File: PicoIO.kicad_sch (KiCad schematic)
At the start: 14 parts

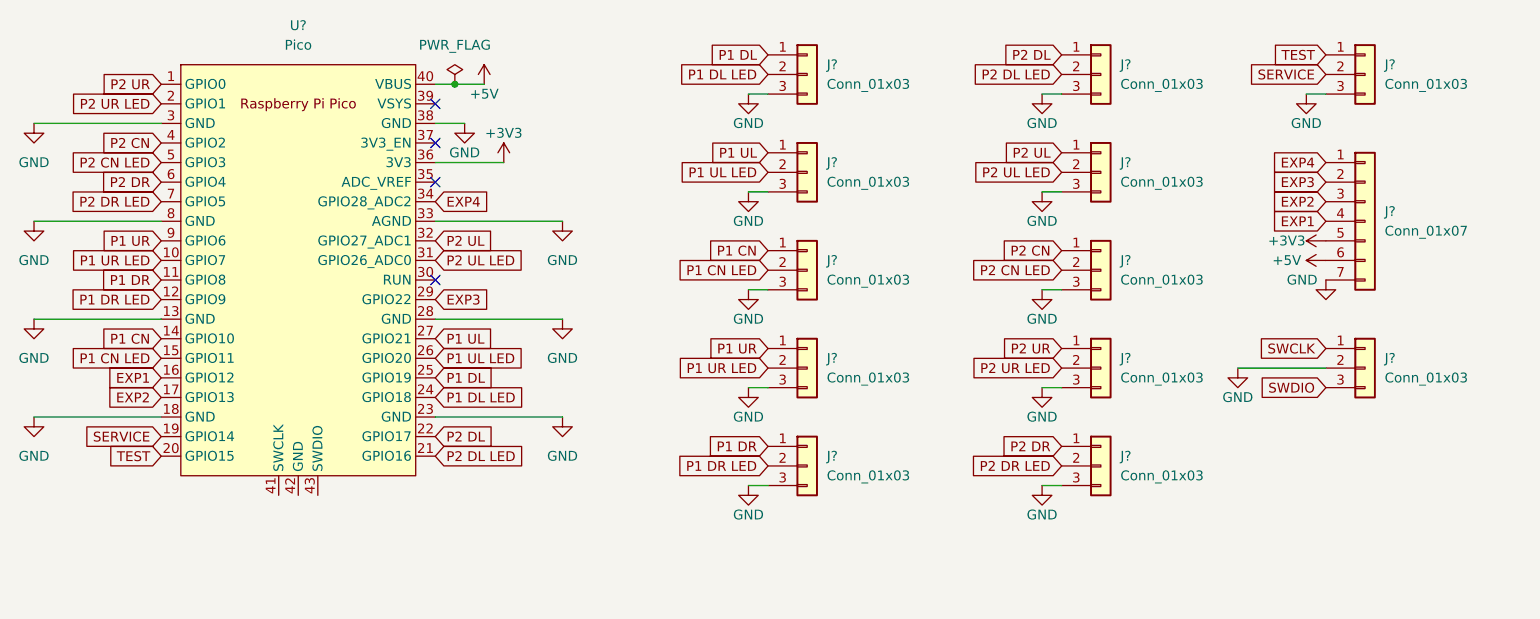
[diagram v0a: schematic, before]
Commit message: PCB revision 1 (NOT READY FOR USE)
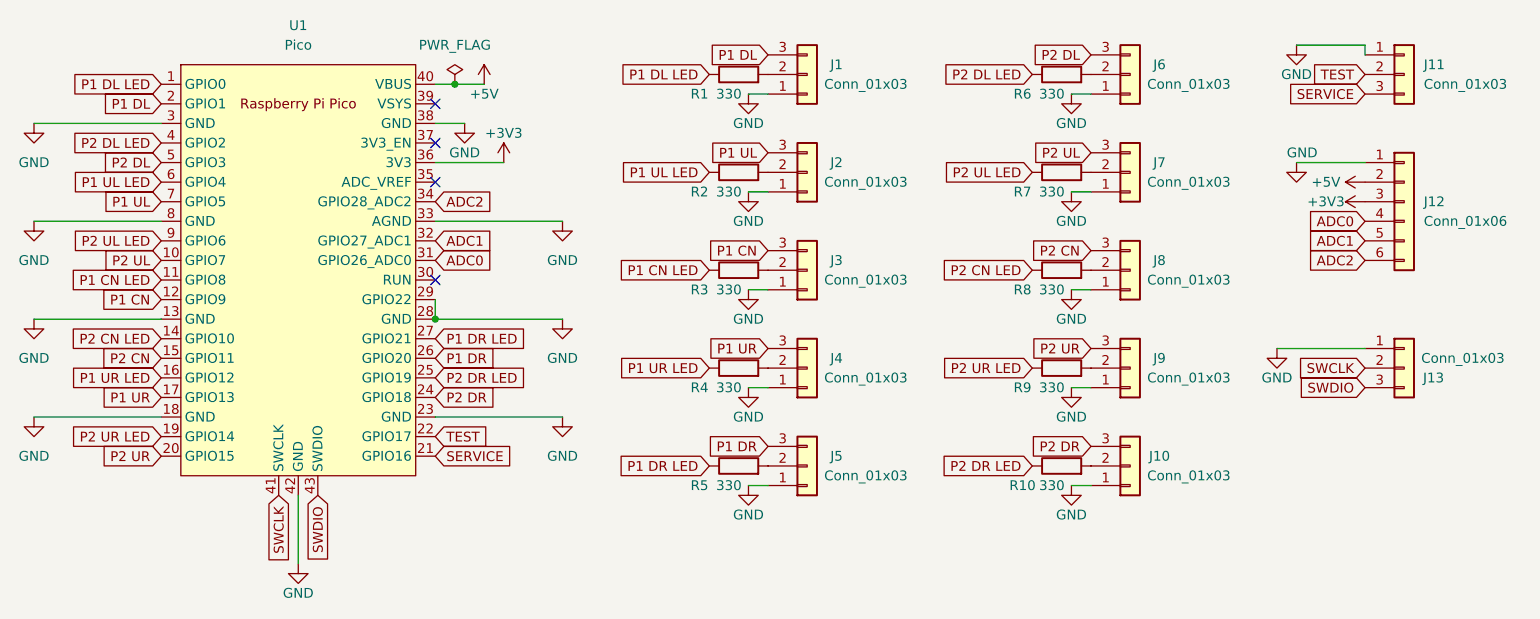
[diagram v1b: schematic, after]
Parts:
- removed J?: Conn_01x07, symbol Connector_Generic:Conn_01x07
- added J12: Conn_01x06, Connector_JST:JST_XH_B6B-XH-A_1x06_P2.50mm_Vertical, symbol Connector_Generic:Conn_01x06
- added R1, R10, R2, R3, R4, R5, R6, R7, R8, R9: 330, Resistor_SMD:R_0805_2012Metric_Pad1.20x1.40mm_HandSolder, symbol Device:R
- J1, J10, J11, J2, J3, J4, J5, J6, J7, J8, J9: renamed from J?; footprint (none) -> Connector_JST:JST_XH_B3B-XH-A_1x03_P2.50mm_Vertical
- J13: renamed from J?; footprint (none) -> Connector_PinHeader_2.54mm:PinHeader_1x03_P2.54mm_Vertical
- U1: renamed from U?; footprint RPi_Pico:RPi_Pico_SMD_TH -> MCU_RaspberryPi_and_Boards:RPi_Pico_SMD_TH
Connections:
- net EXP1 is gone; now on net P1 UR LED: U1.16 (GPIO12)
- net EXP2 is gone; now on net P1 UR: U1.17 (GPIO13)
- net EXP3 is gone; now on net GND: U1.29 (GPIO22)
- net +3V3: now also J12.3 (Pin_3)
- net +5V: now also J12.2 (Pin_2)
- net GND: now also J1.1 (Pin_1), J10.1 (Pin_1), J11.1 (Pin_1), J13.1 (Pin_1), J2.1 (Pin_1), J3.1 (Pin_1), J4.1 (Pin_1), J5.1 (Pin_1), J6.1 (Pin_1), J7.1 (Pin_1), J8.1 (Pin_1), J9.1 (Pin_1), U1.42 (GND), J12.1 (Pin_1); no longer J1.3 (Pin_3), J10.3 (Pin_3), J11.3 (Pin_3), J13.2 (Pin_2), J2.3 (Pin_3), J3.3 (Pin_3), J4.3 (Pin_3), J5.3 (Pin_3), J6.3 (Pin_3), J7.3 (Pin_3), J8.3 (Pin_3), J9.3 (Pin_3)
- net P1 CN: now also J3.3 (Pin_3), U1.12 (GPIO9); no longer J3.1 (Pin_1), U1.14 (GPIO10)
- net P1 CN LED: now also U1.11 (GPIO8), R3.1; no longer J3.2 (Pin_2), U1.15 (GPIO11)
- net P1 DL: now also J1.3 (Pin_3), U1.2 (GPIO1); no longer J1.1 (Pin_1), U1.25 (GPIO19)
- net P1 DL LED: now also U1.1 (GPIO0), R1.1; no longer J1.2 (Pin_2), U1.24 (GPIO18)
- net P1 DR: now also J5.3 (Pin_3), U1.26 (GPIO20); no longer J5.1 (Pin_1), U1.11 (GPIO8)
- net P1 DR LED: now also U1.27 (GPIO21), R5.1; no longer J5.2 (Pin_2), U1.12 (GPIO9)
- net P1 UL: now also J2.3 (Pin_3), U1.7 (GPIO5); no longer J2.1 (Pin_1), U1.27 (GPIO21)
- net P1 UL LED: now also U1.6 (GPIO4), R2.1; no longer J2.2 (Pin_2), U1.26 (GPIO20)
- net P1 UR: now also J4.3 (Pin_3); no longer J4.1 (Pin_1), U1.9 (GPIO6)
- net P1 UR LED: now also R4.1; no longer J4.2 (Pin_2), U1.10 (GPIO7)
- net P2 CN: now also J8.3 (Pin_3), U1.15 (GPIO11); no longer J8.1 (Pin_1), U1.4 (GPIO2)
- net P2 CN LED: now also U1.14 (GPIO10), R8.1; no longer J8.2 (Pin_2), U1.5 (GPIO3)
- net P2 DL: now also J6.3 (Pin_3), U1.5 (GPIO3); no longer J6.1 (Pin_1), U1.22 (GPIO17)
- net P2 DL LED: now also U1.4 (GPIO2), R6.1; no longer J6.2 (Pin_2), U1.21 (GPIO16)
- net P2 DR: now also J10.3 (Pin_3), U1.24 (GPIO18); no longer J10.1 (Pin_1), U1.6 (GPIO4)
- net P2 DR LED: now also U1.25 (GPIO19), R10.1; no longer J10.2 (Pin_2), U1.7 (GPIO5)
- net P2 UL: now also J7.3 (Pin_3), U1.10 (GPIO7); no longer J7.1 (Pin_1), U1.32 (GPIO27_ADC1)
- net P2 UL LED: now also U1.9 (GPIO6), R7.1; no longer J7.2 (Pin_2), U1.31 (GPIO26_ADC0)
- net P2 UR: now also J9.3 (Pin_3), U1.20 (GPIO15); no longer J9.1 (Pin_1), U1.1 (GPIO0)
- net P2 UR LED: now also U1.19 (GPIO14), R9.1; no longer J9.2 (Pin_2), U1.2 (GPIO1)
- net SERVICE: now also J11.3 (Pin_3), U1.21 (GPIO16); no longer J11.2 (Pin_2), U1.19 (GPIO14)
- net SWCLK: now also J13.2 (Pin_2), U1.41 (SWCLK); no longer J13.1 (Pin_1)
- net SWDIO: now also U1.43 (SWDIO)
- net TEST: now also J11.2 (Pin_2), U1.22 (GPIO17); no longer J11.1 (Pin_1), U1.20 (GPIO15)
- net EXP4 renamed ADC2
- net ADC2: now also J12.6 (Pin_6)
- new net: J8.2 (Pin_2), R8.2
- new net: J5.2 (Pin_2), R5.2
- new net: J7.2 (Pin_2), R7.2
- new net: J4.2 (Pin_2), R4.2
- new net: J10.2 (Pin_2), R10.2
- new net: J9.2 (Pin_2), R9.2
- new net: J6.2 (Pin_2), R6.2
- new net: J3.2 (Pin_2), R3.2
- new net: J1.2 (Pin_2), R1.2
- new net: J2.2 (Pin_2), R2.2
- new net ADC0: J12.4 (Pin_4), U1.31 (GPIO26_ADC0)
- new net ADC1: J12.5 (Pin_5), U1.32 (GPIO27_ADC1)
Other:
- moved on the sheet: J10, J11, J13, J6, J7, J8, J9
